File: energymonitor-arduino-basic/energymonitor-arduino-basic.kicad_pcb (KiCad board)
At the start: 2 copper layers, 13 parts, among them J1 Barrel_Jack, J3 Conn_01x04_Male, J4 Conn_01x03_Female, U1 LM358

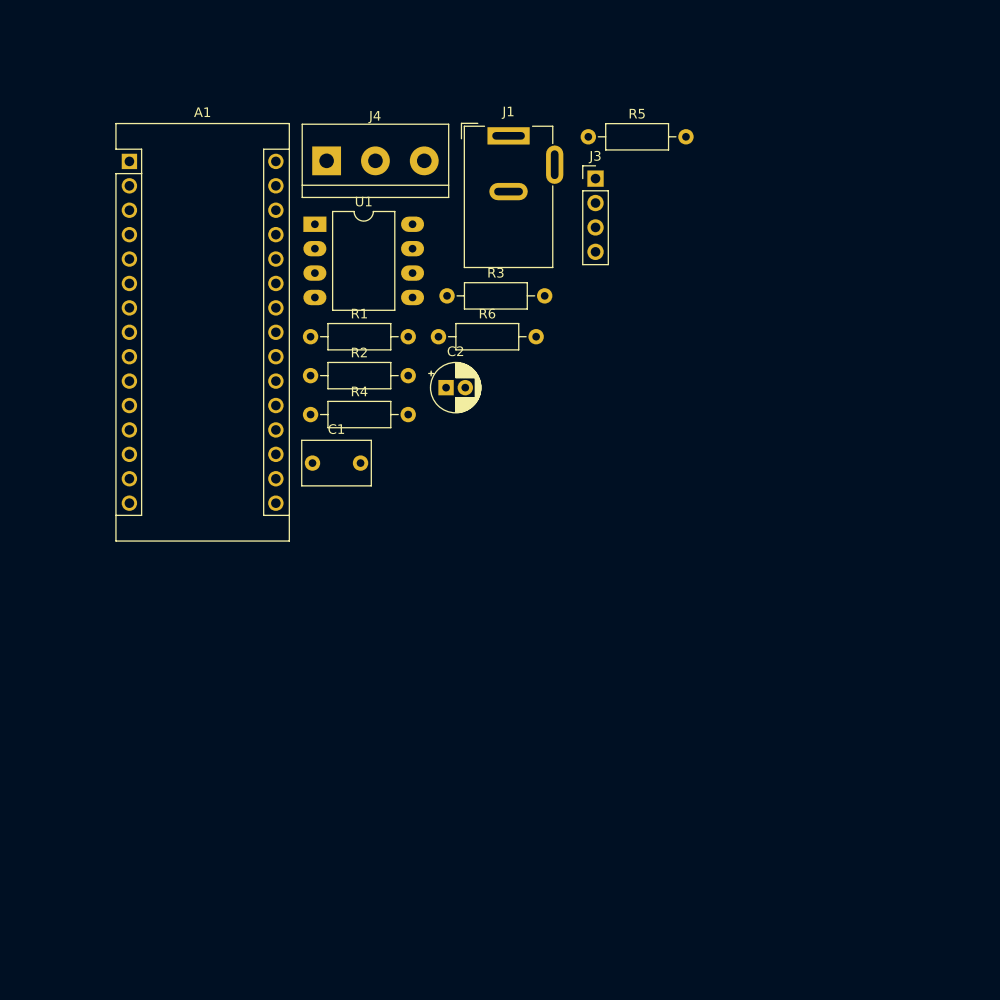
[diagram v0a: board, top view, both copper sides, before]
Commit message: Add some pcb layout
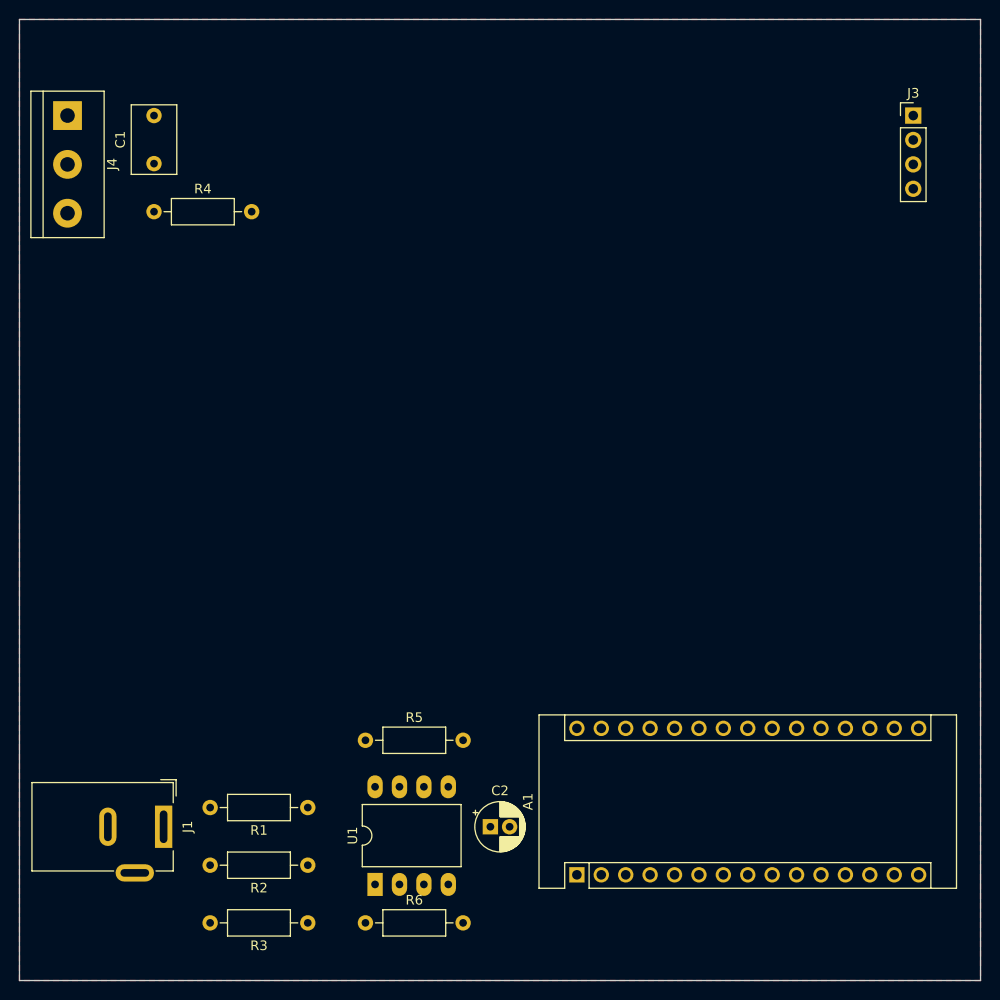
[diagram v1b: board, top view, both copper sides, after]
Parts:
- moved A1 87.6 mm to (138.0, 139.0), turned to 90 degrees
- moved J1 80.4 mm to (95.0, 134.0), turned to 270 degrees
- moved U1 69.0 mm to (117.0, 140.0), turned to 90 degrees
- moved R5 66.9 mm to (116.0, 125.0)
- moved R3 66.8 mm to (110.0, 144.0), turned to 180 degrees
- moved R6 61.5 mm to (116.0, 144.0)
- moved R2 50.9 mm to (110.0, 138.0), turned to 180 degrees
- moved R1 49.0 mm to (110.0, 132.0), turned to 180 degrees
- moved C2 45.9 mm to (129.0, 134.0)
- moved C1 35.3 mm to (94.0, 65.0), turned to 90 degrees
- moved J3 33.7 mm to (173.0, 60.0)
- moved J4 27.4 mm to (85.0, 60.0), turned to 270 degrees
- moved R4 26.7 mm to (94.0, 70.0)
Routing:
- added copper zone on F.Cu, net GND
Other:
- board outline added: 100 x 100 mm
